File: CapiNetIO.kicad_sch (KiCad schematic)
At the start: 78 parts, among them J1 USB_B_Micro, J2 SWD Prg, J4 USART3, J5 InterPCBBus1, J6 InterPCBBus2, SW1 SW_SPDT, U1 STM32F446RETx, U3 AMS1117-3.3, Y1 16MHz

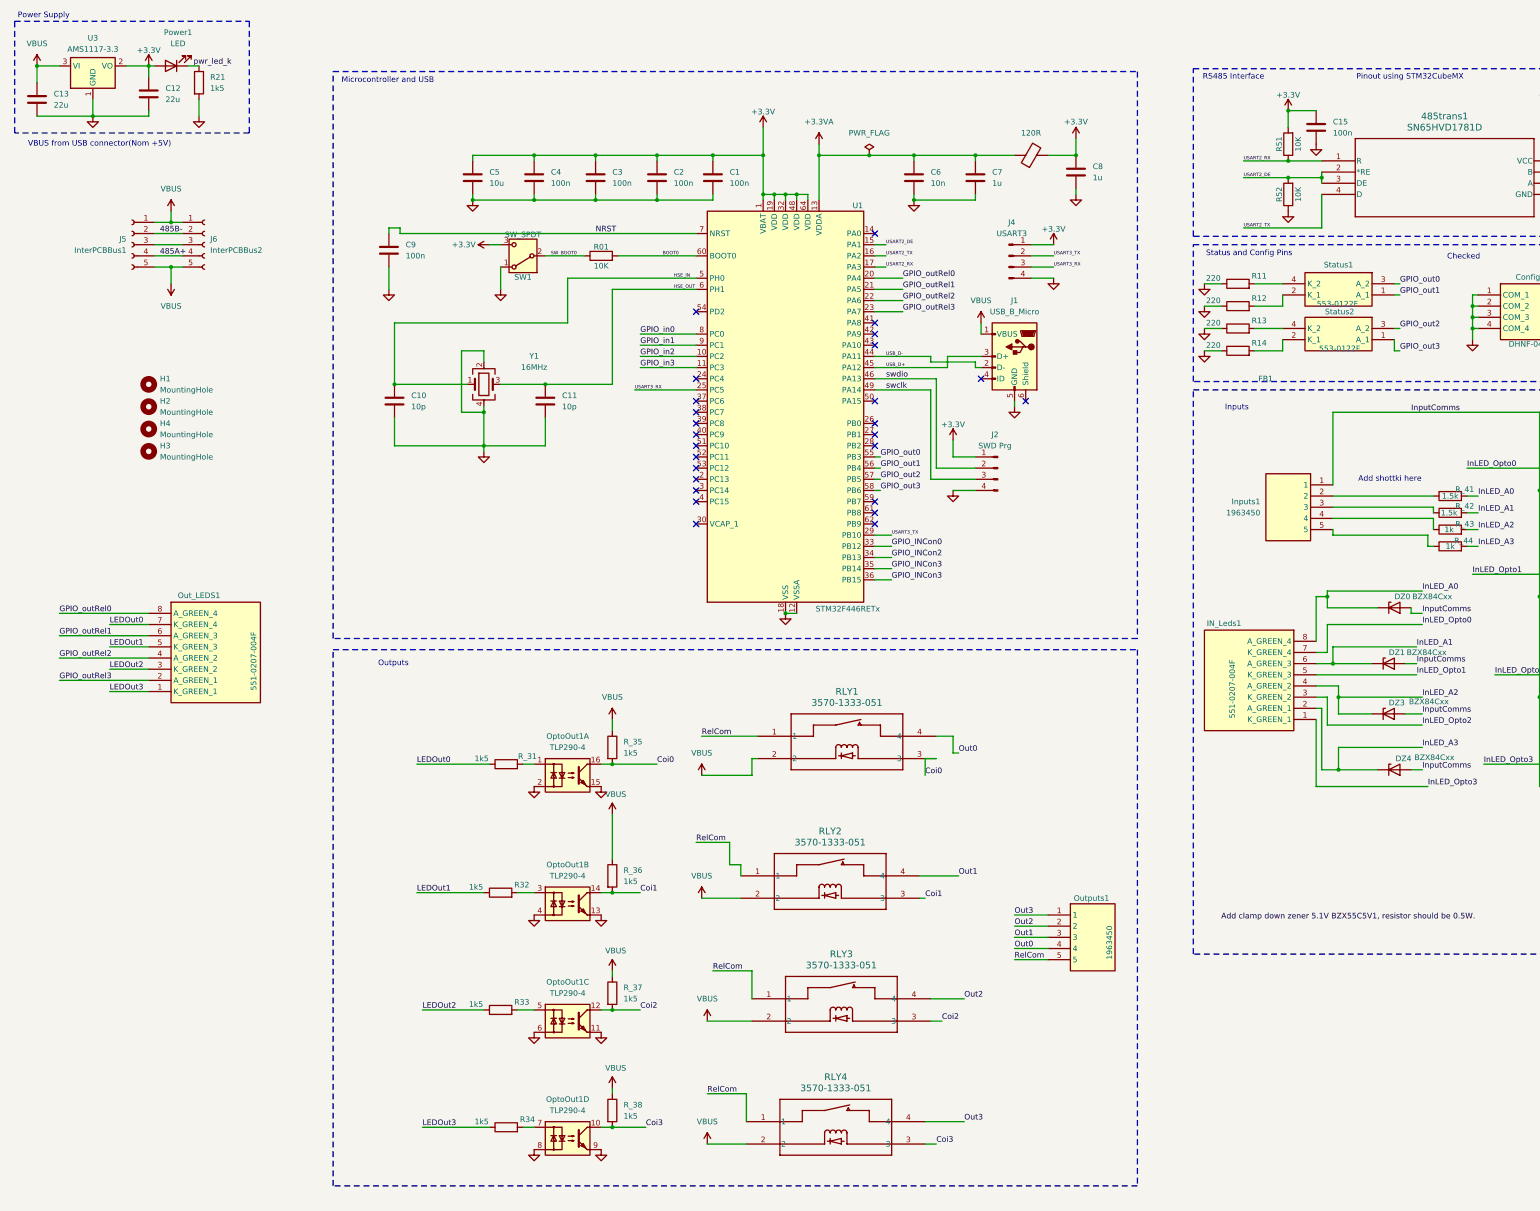
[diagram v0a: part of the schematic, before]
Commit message: checked outputs for resistors and circuits
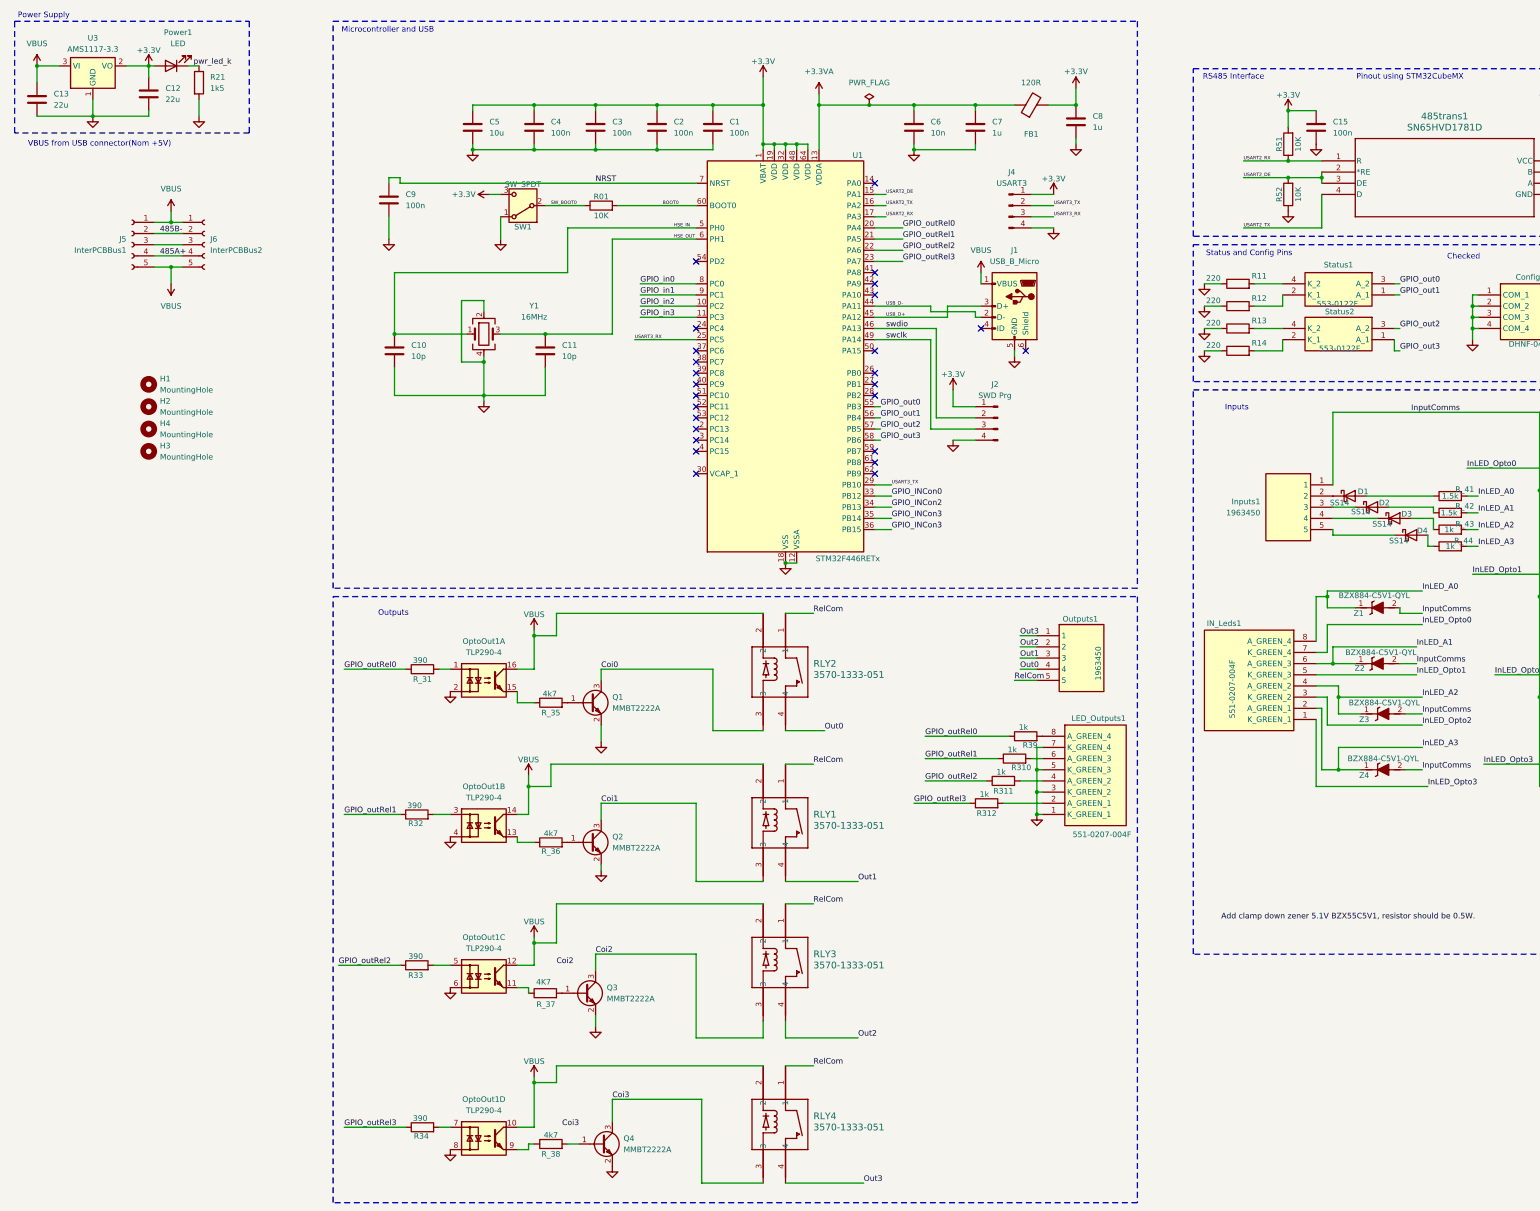
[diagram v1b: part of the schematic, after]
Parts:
- removed DZ0, DZ1, DZ3, DZ4: BZX84Cxx, Package_TO_SOT_SMD:SOT-23, symbol Diode:BZX84Cxx
- removed Out_LEDS1: 551-0207-004F, LED 551 0207 004F:5510207004F, symbol LED Array 551-0207-004F:551-0207-004F
- added D1, D2, D3, D4: SS14, Diode_SMD:D_SMA, symbol Diode:SS14
- added LED_Outputs1: 551-0207-004F, 5510207004F, symbol LED Array 551-0207-004F:551-0207-004F
- added Q1, Q2, Q3, Q4: MMBT2222A, Package_TO_SOT_SMD:SOT-23, symbol Transistor_BJT:MMBT2222A
- added R310, R311, R312, R39: 1k, Resistor_SMD:R_0402_1005Metric, symbol Device:R
- added Z1, Z2, Z3, Z4: BZX884-C5V1-QYL, BZX884C5V1QYL, symbol BZX884-C5V1-QYL_Zener:BZX884-C5V1-QYL
- R32, R33, R34, R_31: value 1k5 -> 390
- RLY1, RLY2, RLY3, RLY4: footprint 3570-1419-054:RELAY4_3570-1333-051_COM -> RELAY4_3570-1333-051_COM
- R_35, R_36, R_38: value 1k5 -> 4k7
- R_37: value 1k5 -> 4K7
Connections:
- net LEDOut0 is gone; now on net GPIO_outRel0: R_31.1
- net LEDOut1 is gone; now on net GPIO_outRel1: R32.1
- net LEDOut2 is gone; now on net GPIO_outRel2: R33.1
- net LEDOut3 is gone; now on net GPIO_outRel3: R34.1
- net Coi0: now also RLY2.3, Q1.3 (C); no longer OptoOut1.16, RLY1.3, R_35.2
- net Coi1: now also RLY1.3, Q2.3 (C); no longer OptoOut1.14, RLY2.3, R_36.2
- net Coi2: now also Q3.3 (C); no longer OptoOut1.12, R_37.2
- net Coi3: now also Q4.3 (C); no longer OptoOut1.10, R_38.2
- net GND: now also LED_Outputs1.1 (K_GREEN_1), LED_Outputs1.3 (K_GREEN_2), LED_Outputs1.5 (K_GREEN_3), LED_Outputs1.7 (K_GREEN_4), Q1.2 (E), Q2.2 (E), Q3.2 (E), Q4.2 (E); no longer OptoOut1.11, OptoOut1.13, OptoOut1.15, OptoOut1.9
- net GPIO_outRel0: now also R39.1
- net GPIO_outRel1: now also R310.1
- net GPIO_outRel2: now also R311.1
- net GPIO_outRel3: now also R312.1
- net InLED_A0: now also Z1.1 (K)
- net InLED_A1: now also Z2.1 (K)
- net InLED_A2: now also Z3.1 (K)
- net InLED_A3: now also Z4.1 (K)
- net InputComms: now also Z1.2 (A), Z2.2 (A), Z3.2 (A), Z4.2 (A)
- net Out0: now also RLY2.4; no longer RLY1.4
- net Out1: now also RLY1.4; no longer RLY2.4
- net VBUS: now also OptoOut1.10, OptoOut1.12, OptoOut1.14, OptoOut1.16; no longer R_35.1, R_36.1, R_37.1, R_38.1
- net at R_43.1: now also D3.2 (A); no longer Inputs1.4
- net at Inputs1.2: now also D1.1 (K); no longer R_41.1
- net at Inputs1.3: now also D2.1 (K); no longer R_42.1
- net at Inputs1.5: now also D4.1 (K); no longer R_44.1
- new net: LED_Outputs1.2 (A_GREEN_1), R312.2
- new net: LED_Outputs1.4 (A_GREEN_2), R311.2
- new net: LED_Outputs1.6 (A_GREEN_3), R310.2
- new net: LED_Outputs1.8 (A_GREEN_4), R39.2
- new net: D2.2 (A), R_42.1
- new net: D3.1 (K), Inputs1.4
- new net: OptoOut1.11, R_37.1
- new net: OptoOut1.9, R_38.1
- new net: Q4.1 (B), R_38.2
- new net: D1.2 (A), R_41.1
- new net: OptoOut1.13, R_36.1
- new net: Q2.1 (B), R_36.2
- new net: D4.2 (A), R_44.1
- new net: Q3.1 (B), R_37.2
- new net: OptoOut1.15, R_35.1
- new net: Q1.1 (B), R_35.2
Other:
- note removed: "Add shottki here"
- moved on the sheet: C1, C10, C11, C2, C3, C4, C5, C6, C7, C8, C9, FB1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
